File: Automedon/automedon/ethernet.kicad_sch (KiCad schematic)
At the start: 3 parts, among them U10 DS108G-M2, U11 ER605v2, U18 OC200

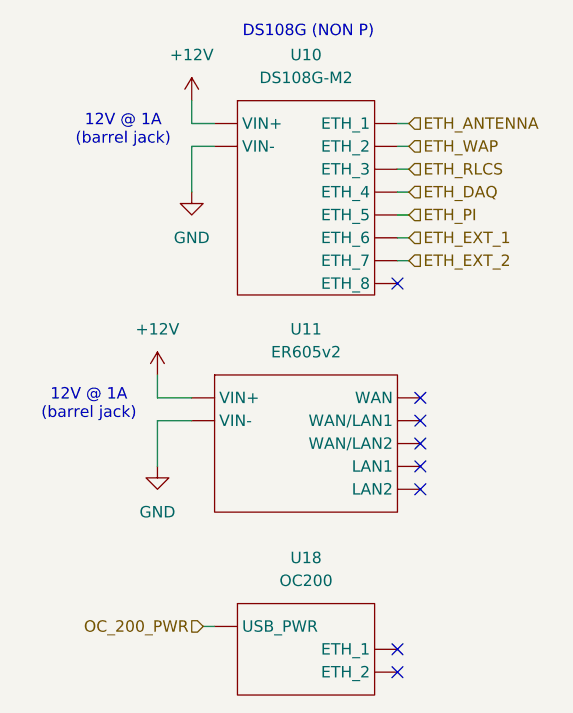
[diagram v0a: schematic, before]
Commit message: Update connector
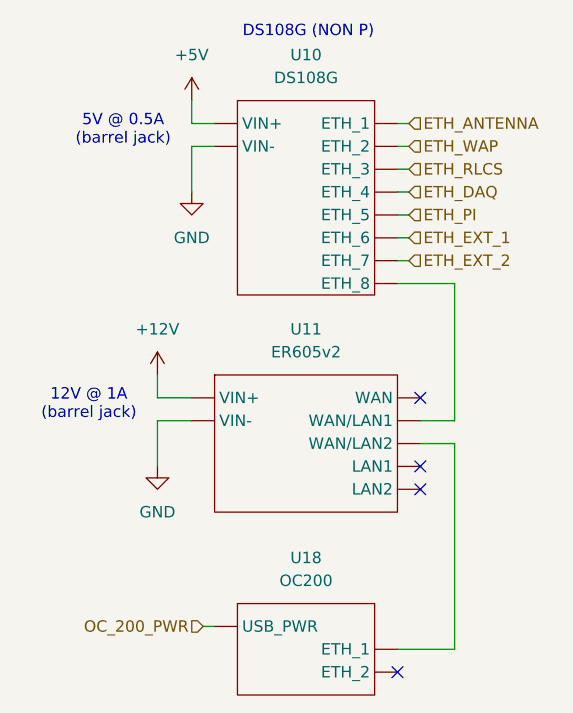
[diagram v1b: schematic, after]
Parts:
- U10: value DS108G-M2 -> DS108G
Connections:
- net +12V: no longer U10. (ETH_8)
- new net: U11. (LAN2), U18. (ETH_2)
- new net: U10. (ETH_8), U11. (LAN2)
- new net +5V: U10. (ETH_8)
- no-connect marks 8 -> 4
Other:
- note added: "5V @ 0.5A (barrel jack)"
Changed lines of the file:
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@@
 	(generator_version "9.0")
 	(paper "A4")
-	(text "12V @ 1A \n(barrel jack)"
+	(text "5V @ 0.5A \n(barrel jack)"
 		(exclude_from_sim no)
 		(at 132.08 70.612 0)
@@
 	)
 	(no_connect
-		(at 162.56 128.27)
-	)
-	(no_connect
 		(at 165.1 107.95)
 	)
@@
 	)
 	(no_connect
-		(at 162.56 87.63)
-	)
-	(no_connect
 		(at 162.56 130.81)
 	)
-	(no_connect
-		(at 165.1 105.41)
-	)
-	(no_connect
-		(at 165.1 102.87)
-	)
 	(wire
 		(pts
@@
 	(wire
 		(pts
+			(xy 165.1 105.41) (xy 168.91 105.41)
+		)
+		(stroke
+			(width 0)
+			(type default)
+		)
+	)
+	(wire
+		(pts
+			(xy 168.91 105.41) (xy 168.91 128.27)
+		)
+		(stroke
+			(width 0)
+			(type default)
+		)
+	)
+	(wire
+		(pts
 			(xy 139.7 69.85) (xy 139.7 67.31)
 		)
@@
 	(wire
 		(pts
+			(xy 162.56 87.63) (xy 168.91 87.63)
+		)
+		(stroke
+			(width 0)
+			(type default)
+		)
+	)
+	(wire
+		(pts
 			(xy 139.7 72.39) (xy 142.24 72.39)
 		)
@@
 	(wire
 		(pts
+			(xy 168.91 87.63) (xy 168.91 102.87)
+		)
+		(stroke
+			(width 0)
+			(type default)
+		)
+	)
+	(wire
+		(pts
 			(xy 139.7 69.85) (xy 142.24 69.85)
+		)
+		(stroke
+			(width 0)
+			(type default)
+		)
+	)
+	(wire
+		(pts
+			(xy 168.91 128.27) (xy 162.56 128.27)
+		)
+		(stroke
+			(width 0)
+			(type default)
+		)
+	)
+	(wire
+		(pts
+			(xy 168.91 102.87) (xy 165.1 102.87)
 		)
 		(stroke
@@
 	)
 	(symbol
-		(lib_id "power:+12V")
+		(lib_id "automedon:ETH_SW")
+		(at 152.4 64.77 0)
+		(unit 1)
+		(exclude_from_sim no)
+		(in_bom yes)
+		(on_board yes)
+		(dnp no)
+		(fields_autoplaced yes)
+		(property "Reference" "U10"
+			(at 152.4 62.23 0)
+			(effects
+				(font
+					(size 1.27 1.27)
+				)
+			)
+		)
+		(property "Value" "DS108G"
+			(at 152.4 64.77 0)
+			(effects
+				(font
+					(size 1.27 1.27)
+				)
+			)
+		)
+		(property "Footprint" ""
+			(at 152.4 64.77 0)
+			(effects
+				(font
+					(size 1.27 1.27)
+				)
+				(hide yes)
+			)
+		)
+		(property "Datasheet" ""
+			(at 152.4 64.77 0)
+			(effects
+				(font
+					(size 1.27 1.27)
+				)
+				(hide yes)
+			)
+		)
+		(property "Description" ""
+			(at 152.4 64.77 0)
+			(effects
+				(font
+					(size 1.27 1.27)
+				)
+				(hide yes)
+			)
+		)
+		(pin ""
+		)
+		(pin ""
+		)
+		(pin ""
+		)
+		(pin ""
+		)
+		(pin ""
+		)
+		(pin ""
+		)
+		(pin ""
+		)
+		(pin ""
+		)
+		(pin ""
+		)
+		(pin ""
+		)
+		(instances
+			(project ""
+				(path "/75831ec5-d9f4-4d6d-a97b-0bb87f785768/a01756e2-dff9-4d90-8b5d-2eadc2973bae"
+					(reference "U10")
+					(unit 1)
+				)
+			)
+		)
+	)
+	(symbol
+		(lib_id "power:GND")
+		(at 139.7 77.47 0)
+		(unit 1)
+		(exclude_from_sim no)
+		(in_bom yes)
+		(on_board yes)
+		(dnp no)
+		(fields_autoplaced yes)
+		(property "Reference" "#PWR020"
+			(at 139.7 83.82 0)
+			(effects
+				(font
+					(size 1.27 1.27)
+				)
+				(hide yes)
+			)
+		)
+		(property "Value" "GND"
+			(at 139.7 82.55 0)
+			(effects
+				(font
+					(size 1.27 1.27)
+				)
+			)
+		)
+		(property "Footprint" ""
+			(at 139.7 77.47 0)
+			(effects
+				(font
+					(size 1.27 1.27)
+				)
+				(hide yes)
+			)
+		)
+		(property "Datasheet" ""
+			(at 139.7 77.47 0)
+			(effects
+				(font
+					(size 1.27 1.27)
+				)
+				(hide yes)
+			)
+		)
+		(property "Description" "Power symbol creates a global label with name \"GND\" , ground"
+			(at 139.7 77.47 0)
+			(effects
+				(font
+					(size 1.27 1.27)
+				)
+				(hide yes)
+			)
+		)
+		(pin "1"
+		)
+		(instances
+			(project ""
+				(path "/75831ec5-d9f4-4d6d-a97b-0bb87f785768/a01756e2-dff9-4d90-8b5d-2eadc2973bae"
+					(reference "#PWR020")
+					(unit 1)
+				)
+			)
+		)
+	)
+	(symbol
+		(lib_id "power:+5V")
 		(at 139.7 67.31 0)
 		(unit 1)
@@
 			)
 		)
-		(property "Value" "+12V"
+		(property "Value" "+5V"
 			(at 139.7 62.23 0)
 			(effects
@@
 			)
 		)
-		(property "Description" "Power symbol creates a global label with name \"+12V\""
+		(property "Description" "Power symbol creates a global label with name \"+5V\""
 			(at 139.7 67.31 0)
 			(effects
@@
 					(unit 1)
 				)
-			)
-		)
-	)
-	(symbol
-		(lib_id "automedon:ETH_SW")
-		(at 152.4 64.77 0)
-		(unit 1)
-		(exclude_from_sim no)
-		(in_bom yes)
-		(on_board yes)
-		(dnp no)
-		(fields_autoplaced yes)
-		(property "Reference" "U10"
-			(at 152.4 62.23 0)
-			(effects
-				(font
-					(size 1.27 1.27)
-				)
-			)
-		)
-		(property "Value" "DS108G-M2"
-			(at 152.4 64.77 0)
-			(effects
-				(font
-					(size 1.27 1.27)
-				)
-			)
-		)
-		(property "Footprint" ""
-			(at 152.4 64.77 0)
-			(effects
-				(font
-					(size 1.27 1.27)
-				)
-				(hide yes)
-			)
-		)
-		(property "Datasheet" ""
-			(at 152.4 64.77 0)
-			(effects
-				(font
-					(size 1.27 1.27)
-				)
-				(hide yes)
-			)
-		)
-		(property "Description" ""
-			(at 152.4 64.77 0)
-			(effects
-				(font
-					(size 1.27 1.27)
-				)
-				(hide yes)
-			)
-		)
-		(pin ""
-		)
-		(pin ""
-		)
-		(pin ""
-		)
-		(pin ""
-		)
-		(pin ""
-		)
-		(pin ""
-		)
-		(pin ""
-		)
-		(pin ""
-		)
-		(pin ""
-		)
-		(pin ""
-		)
-		(instances
-			(project ""
-				(path "/75831ec5-d9f4-4d6d-a97b-0bb87f785768/a01756e2-dff9-4d90-8b5d-2eadc2973bae"
-					(reference "U10")
-					(unit 1)
-				)
-			)
-		)
-	)
-	(symbol
-		(lib_id "power:GND")
-		(at 139.7 77.47 0)
-		(unit 1)
-		(exclude_from_sim no)
-		(in_bom yes)
-		(on_board yes)
-		(dnp no)
-		(fields_autoplaced yes)
-		(property "Reference" "#PWR020"
-			(at 139.7 83.82 0)
-			(effects
-				(font
-					(size 1.27 1.27)
-				)
-				(hide yes)
-			)
-		)
-		(property "Value" "GND"
-			(at 139.7 82.55 0)
-			(effects
-				(font
-					(size 1.27 1.27)
-				)
-			)
-		)
-		(property "Footprint" ""
-			(at 139.7 77.47 0)
-			(effects
-				(font
-					(size 1.27 1.27)
-				)
-				(hide yes)
-			)
-		)
-		(property "Datasheet" ""
-			(at 139.7 77.47 0)
-			(effects
-				(font
-					(size 1.27 1.27)
-				)
-				(hide yes)
-			)
-		)
-		(property "Description" "Power symbol creates a global label with name \"GND\" , ground"
-			(at 139.7 77.47 0)
-			(effects
-				(font
-					(size 1.27 1.27)
-				)
-				(hide yes)
-			)
-		)
-		(pin "1"
-		)
-		(instances
-			(project ""
-				(path "/75831ec5-d9f4-4d6d-a97b-0bb87f785768/a01756e2-dff9-4d90-8b5d-2eadc2973bae"
-					(reference "#PWR020")
-					(unit 1)
-				)
